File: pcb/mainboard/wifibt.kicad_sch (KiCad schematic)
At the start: 11 parts, among them U901 RTL8723BS

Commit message: - pcb: start r0p1 layout
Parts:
- R902: footprint Resistor_SMD:R_0603_1608Metric -> Resistor_SMD:R_0402_1005Metric
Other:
- company: Copyright EI-2030 2021. -> Copyright EI-2030 2021. / Engineer: Wenting Zhang
- title: Archer -> Archer Mainboard
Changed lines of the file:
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@@
   (paper "A3")
   (title_block
-    (title "Archer")
-    (date "2021-04-26")
+    (title "Archer Mainboard")
+    (date "2021-05-05")
     (rev "R0.1 draft")
-    (company "Copyright EI-2030 2021.")
+    (company "Copyright EI-2030 2021. / Engineer: Wenting Zhang")
     (comment 2 "MERCHANTABILITY, SATISFACTORY QUALITY AND FITNESS FOR A PARTICULAR PURPOSE.")
-    (comment 3 "source is distributed WITHOUT ANY EXPRESS OR IMPLIED WARRANTY, INCLUDING OF")
-    (comment 4 "This source describes Open Hardware and is licensed under the CERN-OHL-S v2. This ")
+    (comment 3 "This source is distributed WITHOUT ANY EXPRESS OR IMPLIED WARRANTY, INCLUDING OF")
+    (comment 4 "This source describes Open Hardware and is licensed under the CERN-OHL-S v2.")
   )
   (junction (at 109.22 134.62) (diameter 0.9144) (color 0 0 0 0))
@@
       (effects (font (size 1.27 1.27)) (justify left))
     )
-    (property "Footprint" "Resistor_SMD:R_0603_1608Metric" (id 2) (at 132.842 69.85 90)
-      (effects (font (size 1.27 1.27)) hide)
-    )
+    (property "Footprint" "Resistor_SMD:R_0402_1005Metric" (id 2) (at 132.842 69.85 90)
+      (effects (font (size 1.27 1.27)) hide)
+    )

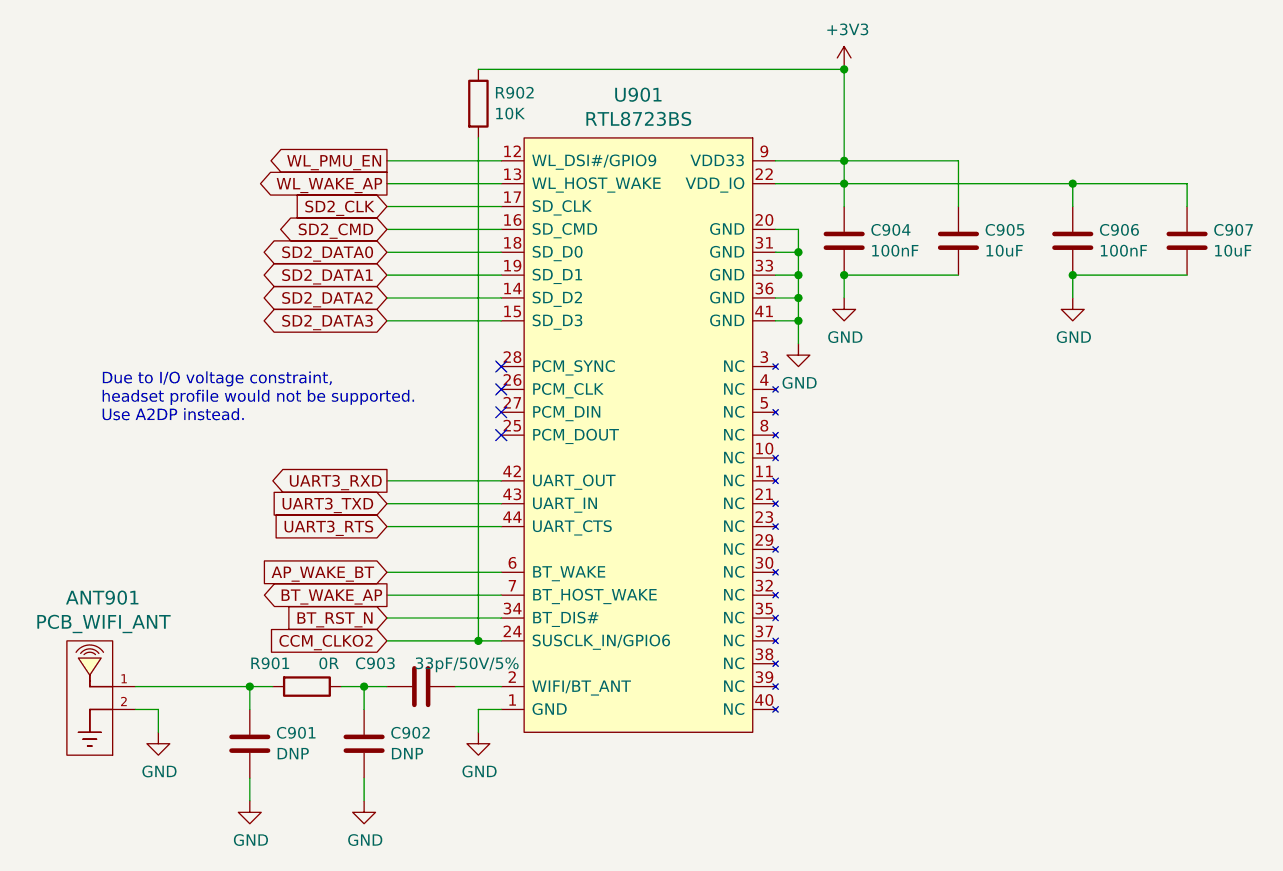
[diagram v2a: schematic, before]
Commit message: - pcb: finishing layout r0p1
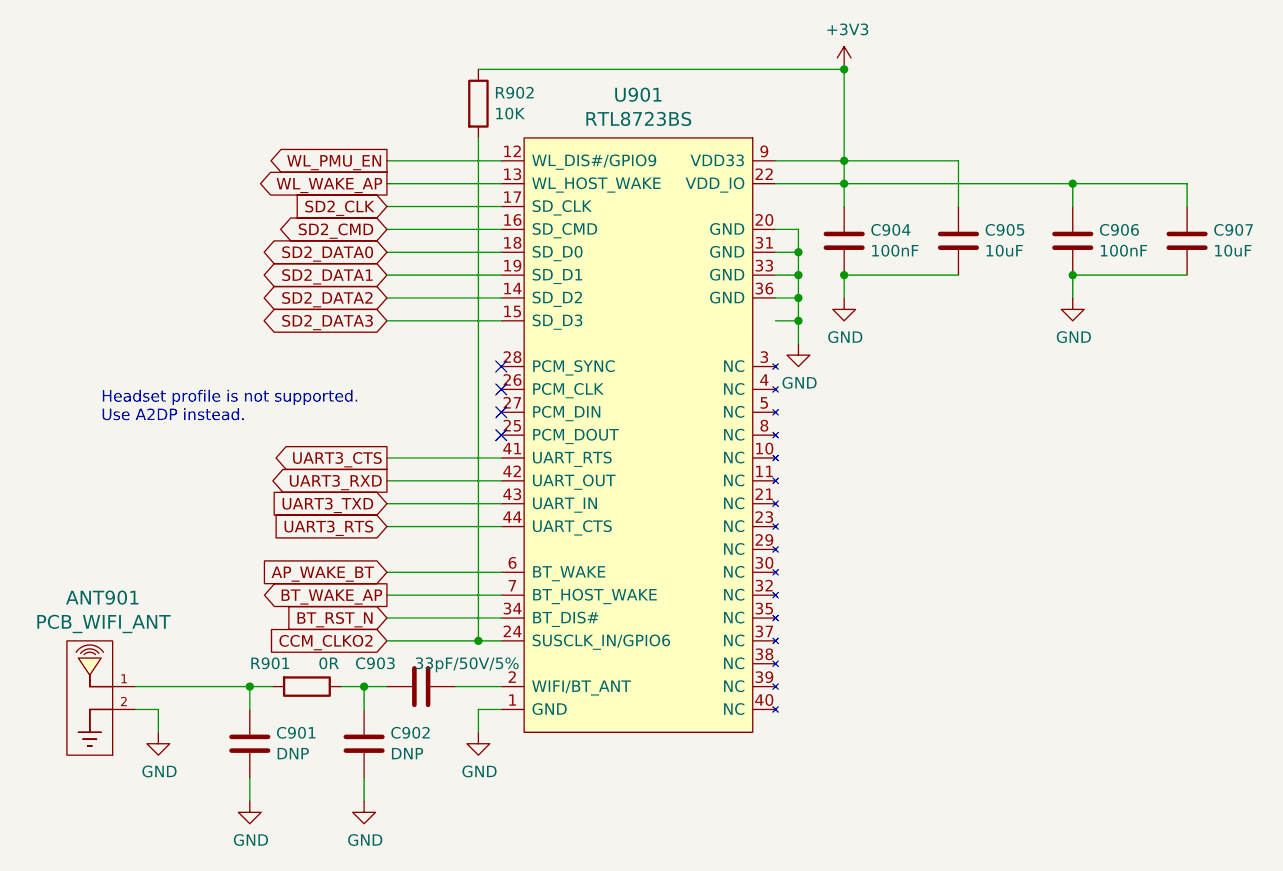
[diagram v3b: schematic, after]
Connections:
- net GND: no longer U901.41 (GND)
- new net UART3_CTS: U901.41 (UART_RTS)
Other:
- note added: "Headset profile is not supported. Use A2DP instead."
- note removed: "Due to I/O voltage constraint, headset profile would not be supported. Use A2DP instead."
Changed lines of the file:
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@@
+    (stroke (width 0) (type solid) (color 0 0 0 0))
+  )
+  (wire (pts (xy 124.46 109.22) (xy 137.16 109.22))
     (stroke (width 0) (type solid) (color 0 0 0 0))
   )
@@
     (stroke (width 0) (type solid) (color 0 0 0 0))
   )
-  (text "Due to I/O voltage constraint,\nheadset profile would not be supported.\nUse A2DP instead."
+  (text "Headset profile is not supported.\nUse A2DP instead."
     (at 92.71 105.41 0)
     (effects (font (size 1.27 1.27)) (justify left bottom))
@@
     )
   )
+  (global_label "UART3_CTS" (shape output) (at 124.46 109.22 180) (fields_autoplaced)
+    (effects (font (size 1.27 1.27)) (justify right))
+    (property "Intersheet References" "${INTERSHEET_REFS}" (id 0) (at 111.7659 109.1406 0)
+      (effects (font (size 1.27 1.27)) (justify right) hide)
+    )
+  )
